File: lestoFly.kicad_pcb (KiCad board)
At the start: 2 copper layers, 36 x 36 mm, 25 parts, among them J1 Conn_01x02_Male, J2 Conn_01x04_Male, J3 Conn_01x05_Male, J4 Conn_01x03_Male, J5 Conn_Coaxial, U1 ESP32-WROOM-32D, U2 LMZM23601V3, U3 BMP280, U4 RFM95W-868S2, U5 BMX160

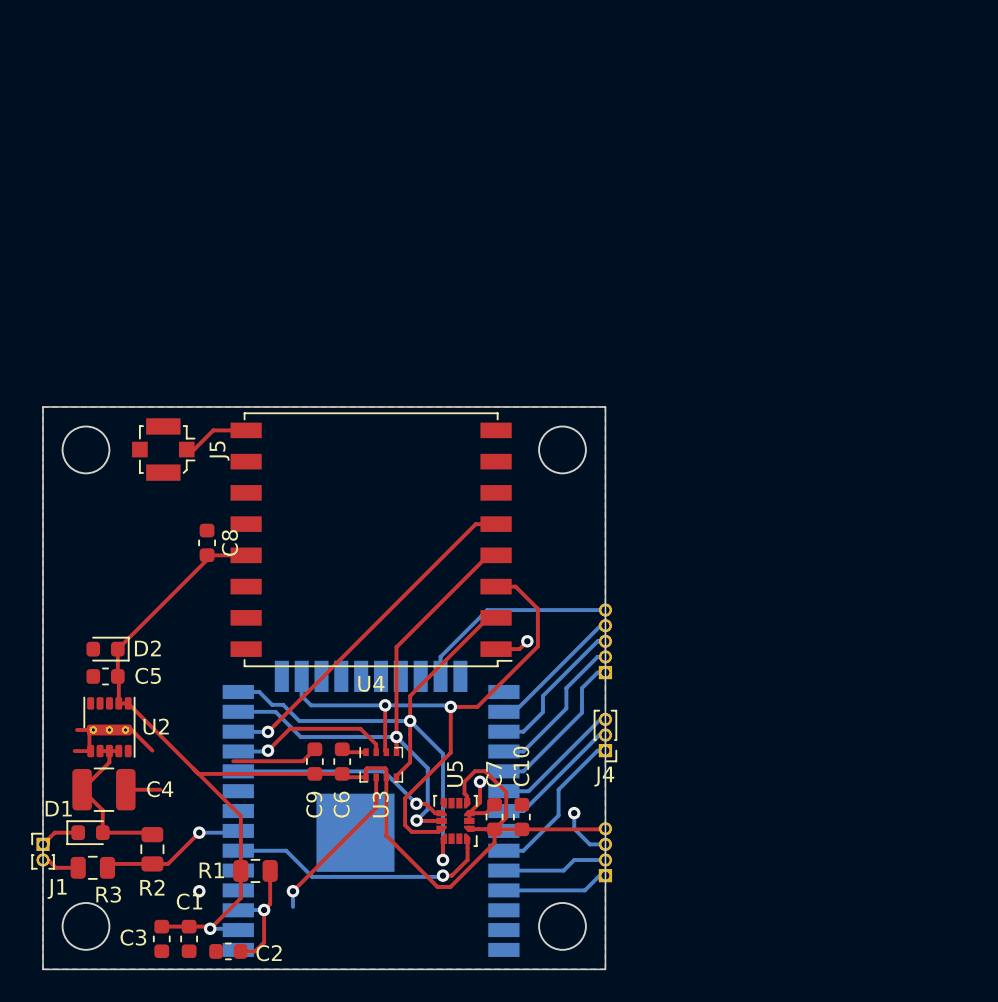
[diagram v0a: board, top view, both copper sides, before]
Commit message: board pcb redraw
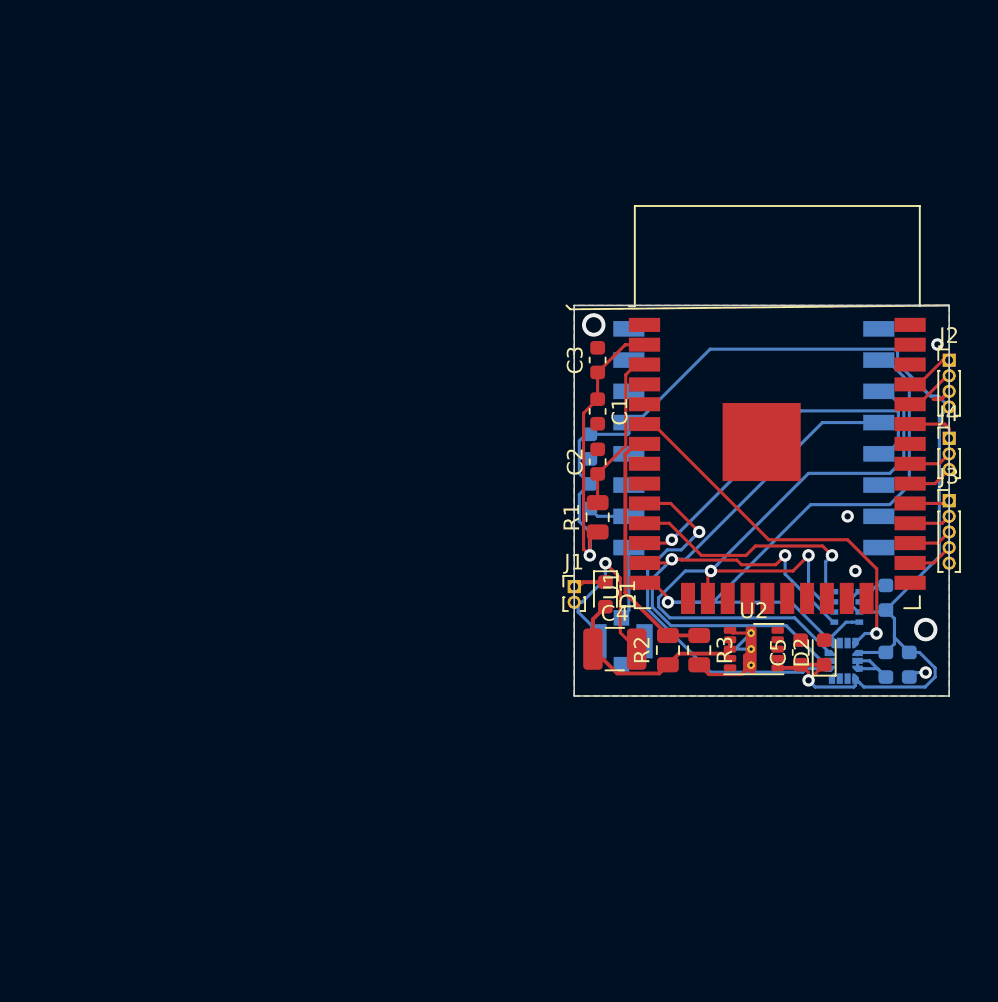
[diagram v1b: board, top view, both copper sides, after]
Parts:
- C10, C6, C7, C8, C9, J5, U3, U4, U5: moved to B.Cu
- J2, J3, U1: moved to F.Cu
- moved C3 46.4 mm to (99.5, 61.0), turned to 90 degrees
- moved D2 46.0 mm to (114.0, 79.7), turned to 90 degrees
- moved C5 44.5 mm to (112.5, 79.7), turned to 90 degrees
- moved C8 43.6 mm to (118.0, 76.2)
- moved C1 42.7 mm to (99.5, 64.3)
- moved U2 41.6 mm to (109.5, 79.5), turned to 0 degrees
- moved R3 41.2 mm to (106.0, 79.6), turned to 270 degrees
- moved J2 39.7 mm to (122.0, 61.0)
- moved C2 39.3 mm to (99.5, 67.5), turned to 90 degrees
- moved J1 37.8 mm to (98.0, 75.5)
- moved D1 36.3 mm to (100.0, 76.0), turned to 270 degrees
- moved R2 35.4 mm to (104.0, 79.6), turned to 90 degrees
- moved U1 35.0 mm to (111.0, 67.0)
- moved C4 33.9 mm to (100.6, 79.5)
- moved J5 31.8 mm to (101.0, 79.0), turned to 0 degrees
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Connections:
- U1 pad 23: Net-(J3-Pad5) -> Net-(U1-Pad23)
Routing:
- net +3V3: track 81.9 -> 98.7 mm, vias 1 -> 2
- net CLK: track 34.4 -> 48.4 mm
- net Net-(J3-Pad5): track 12.7 -> 0.00 mm
- net MOSI: track 38.3 -> 50.3 mm
- net CS_IMU: track 14.1 -> 24.5 mm
- net MISO: track 35.7 -> 44.5 mm, vias 2 -> 1
- net INT_IMU: track 17.2 -> 24.4 mm
- net Net-(J3-Pad1): track 9.72 -> 2.57 mm
- net BAT_SCALED: track 9.35 -> 16.2 mm, vias 1 -> 0
- net Net-(J3-Pad2): track 9.45 -> 2.68 mm
- net Net-(J4-Pad1): track 9.80 -> 3.24 mm
- net Net-(J3-Pad3): track 9.18 -> 2.80 mm
- net CS_BARO: track 10.4 -> 16.8 mm
- net Net-(J3-Pad4): track 8.47 -> 2.91 mm
- net Net-(J4-Pad2): track 8.19 -> 2.76 mm
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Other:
- board size 36 x 36 mm -> 24 x 25 mm
- net class Default: clearance 0.15 -> 0.1
- rule trace_clearance: 0.15 -> 0.1

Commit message: new review finish
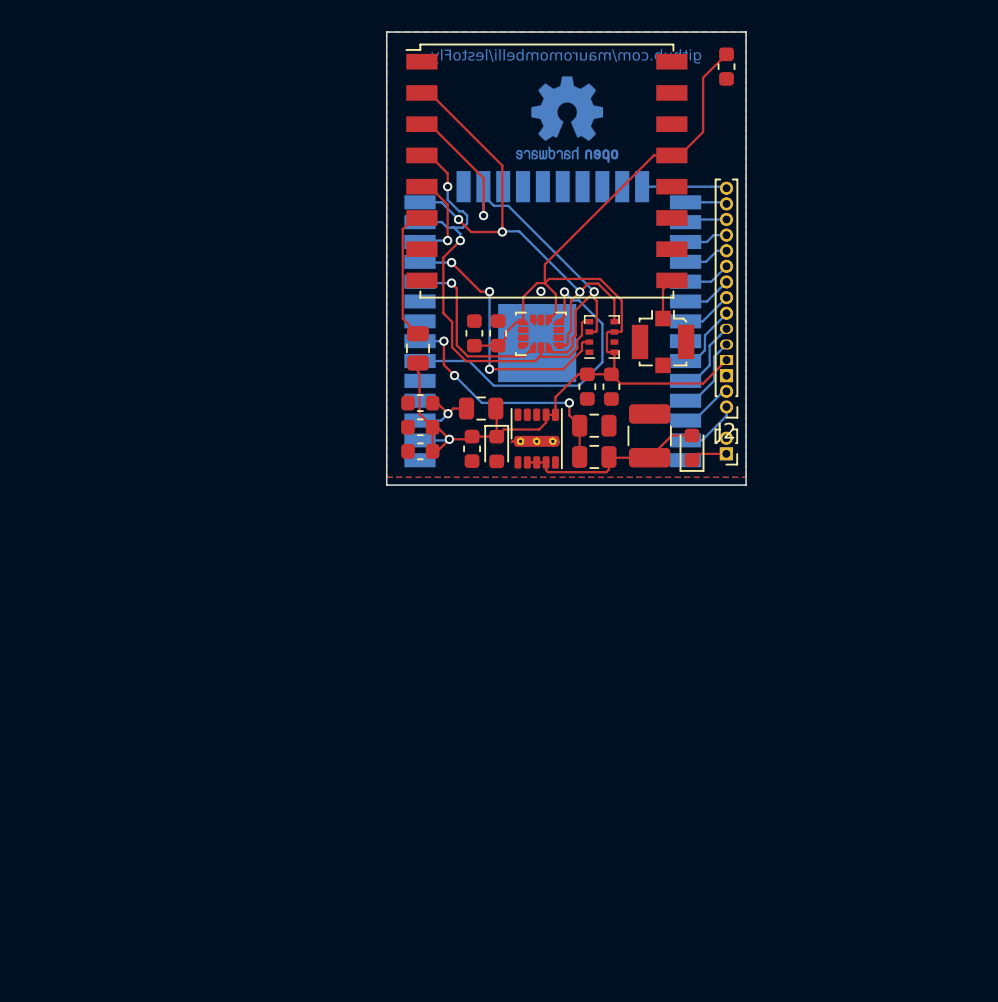
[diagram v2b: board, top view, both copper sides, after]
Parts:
- removed J3: Conn_01x05_Male, Connector_PinHeader_1.00mm:PinHeader_1x05_P1.00mm_Vertical
- removed J4: Conn_01x03_Male, Connector_PinHeader_1.00mm:PinHeader_1x03_P1.00mm_Vertical
- added R4: 10k, Resistor_SMD:R_0805_2012Metric, F.Cu at (88.0, 60.2)
- added REF**: OSHW-Logo2_7.3x6mm_Copper, Symbol:OSHW-Logo2_7.3x6mm_Copper, B.Cu at (97.5, 45.6)
- C10, C6, C7, C8, C9, J5, U3, U4, U5: moved to F.Cu
- J2: value Conn_01x04_Male -> Conn_01x15_Male; footprint Connector_PinHeader_1.00mm:PinHeader_1x04_P1.00mm_Vertical -> Connector_PinHeader_1.00mm:PinHeader_1x15_P1.00mm_Vertical
- U1: moved to B.Cu
- moved C8 35.5 mm to (107.8, 42.2), turned to 270 degrees
- moved C7 33.8 mm to (91.6, 59.3), turned to 90 degrees
- moved C10 33.8 mm to (93.1, 59.3), turned to 90 degrees
- moved U5 28.5 mm to (95.9, 59.3), turned to 180 degrees
- moved C5 24.7 mm to (91.5, 66.7), turned to 270 degrees
- moved D2 24.7 mm to (93.0, 66.7), turned to 270 degrees
- moved U3 23.3 mm to (99.8, 59.5), turned to 90 degrees
- moved U4 21.6 mm to (96.2, 48.9), turned to 0 degrees
- moved U2 19.4 mm to (95.6, 66.0), turned to 90 degrees
- moved J5 19.3 mm to (103.7, 59.8), turned to 180 degrees
- moved U1 16.4 mm to (96.6, 59.2)
- moved R3 15.9 mm to (99.3, 65.2), turned to 0 degrees
- moved J2 14.6 mm to (107.8, 64.0), turned to 180 degrees
- moved C4 13.8 mm to (102.8, 65.8), turned to 90 degrees
- moved R2 13.2 mm to (99.3, 67.2), turned to 180 degrees
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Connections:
- J2 pad 1: Net-(J2-Pad1) -> 1
- J2 pad 2: Net-(J2-Pad2) -> 2
- U1 pad 24: Net-(U1-Pad24) -> 15
- U1 pad 25: Net-(U1-Pad25) -> 14
- U1 pad 26: Net-(J3-Pad4) -> 13
- U1 pad 27: Net-(J3-Pad3) -> 12
- U1 pad 28: Net-(J3-Pad2) -> 11
- U1 pad 29: Net-(J3-Pad1) -> 10
- U1 pad 30: Net-(J4-Pad3) -> 9
- U1 pad 31: Net-(J4-Pad2) -> 8
- U1 pad 33: Net-(J4-Pad1) -> 7
- U1 pad 34: Net-(J2-Pad2) -> 6
- U1 pad 35: Net-(J2-Pad1) -> 5
- U1 pad 36: Net-(U1-Pad36) -> 2
- U1 pad 37: Net-(U1-Pad37) -> 1
- U5 pad 2: Net-(U5-Pad2) -> GND
- U5 pad 3: Net-(U5-Pad3) -> GND
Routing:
- net GND: track 39.7 -> 3.58 mm, vias 5 -> 1
- net +3V3: track 98.7 -> 76.4 mm, vias 2 -> 1
- net MOSI: track 50.3 -> 28.8 mm
- net CLK: track 48.4 -> 29.4 mm
- net CS_LORA: track 23.3 -> 6.23 mm
- net CS_IMU: track 24.5 -> 11.6 mm
- net MISO: track 44.5 -> 32.5 mm, vias 1 -> 3
- net Net-(R4-Pad1): track 0.00 -> 8.62 mm
- net Net-(C2-Pad1): track 10.4 -> 4.56 mm, vias 0 -> 1
- net 15: track 0.00 -> 5.45 mm
- net 5: track 0.00 -> 5.01 mm
- net 6: track 0.00 -> 4.74 mm
- net 7: track 0.00 -> 4.47 mm
- net 1: track 0.00 -> 3.84 mm
- net INT_IMU: track 24.4 -> 20.8 mm
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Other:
- board size 24 x 25 mm -> 23 x 29 mm
- net class Default: clearance 0.1 -> 0.15; trace_width 0.25 -> 0.15; via_dia 0.8 -> 0.6; via_drill 0.4 -> 0.35
- rule trace_clearance: 0.1 -> 0.15
- rule trace_min: 0.2 -> 0.15
- rule via_min_drill: 0.3 -> 0.35
- rule via_min_size: 0.4 -> 0.6
- board text added: "github.com/mauromombelli/lestoFly"
